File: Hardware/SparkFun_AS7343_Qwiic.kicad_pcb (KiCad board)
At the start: 2 copper layers, 25.4 x 25.4 mm, 67 parts, among them J1 Qwiic_RA, J2 Qwiic_RA, J3 Conn_01x06, Q1 BSS138, Q2 BSS138, U1 RT9080-1.8V, U2 AS7343

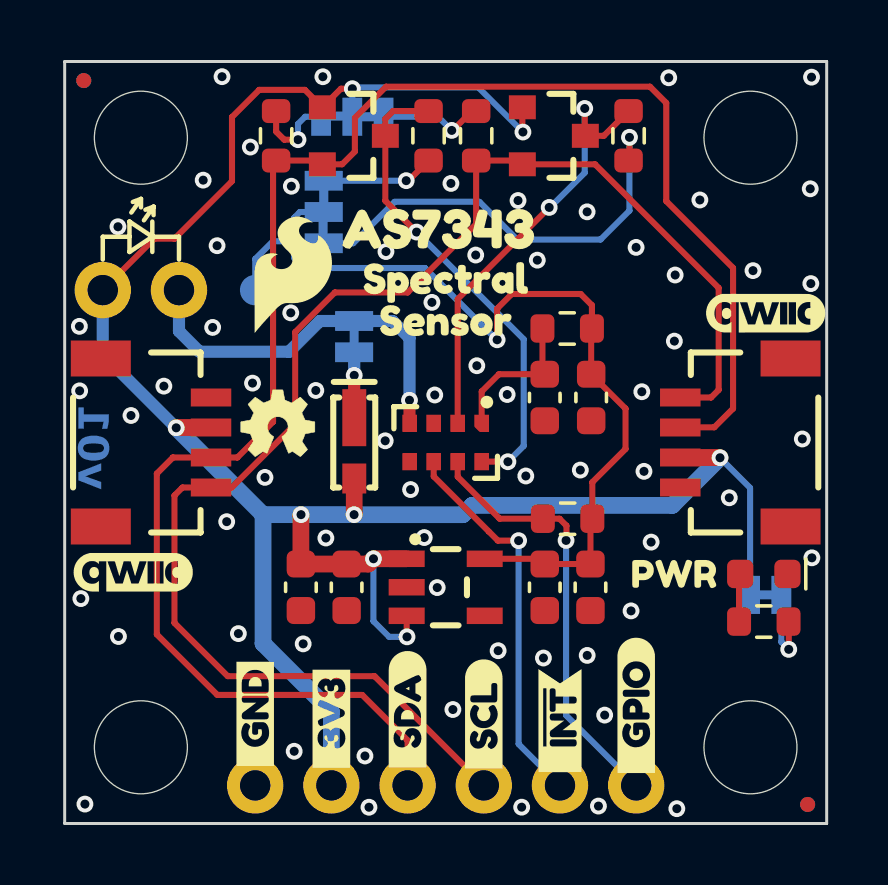
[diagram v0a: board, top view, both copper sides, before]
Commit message: measures
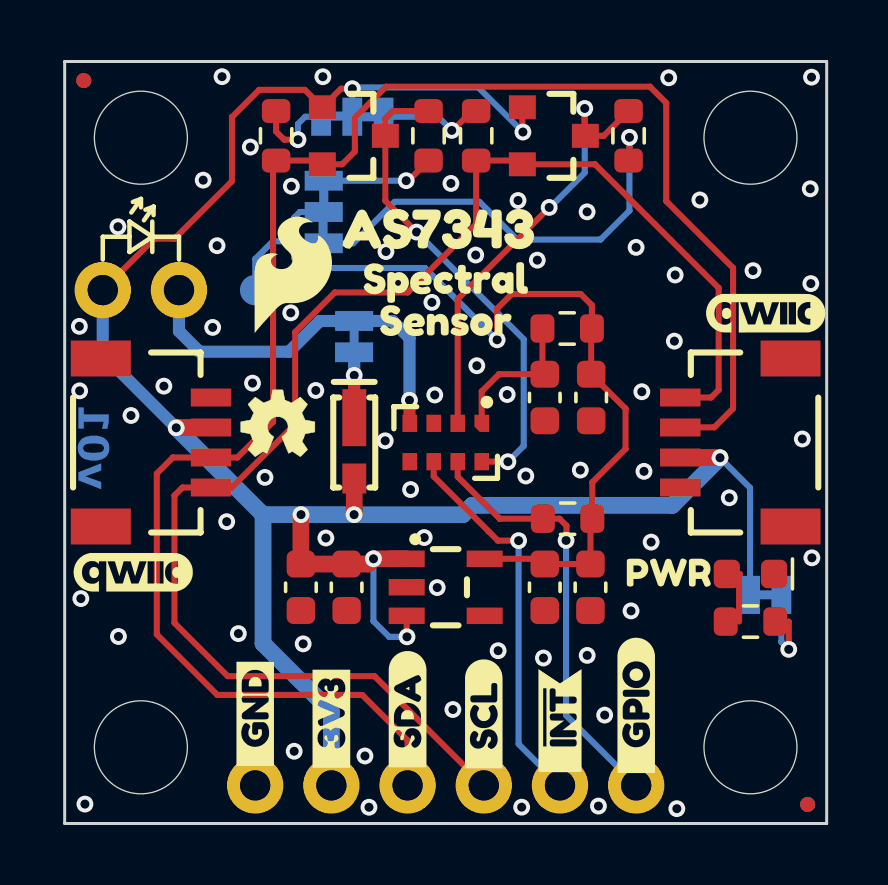
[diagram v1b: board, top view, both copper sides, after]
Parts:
- moved D1 0.44 mm to (146.1, 102.5)
- moved R3 0.44 mm to (146.1, 104.1)
- moved kibuzzard-65A8A8B4 0.19 mm to (143.4, 102.4)
